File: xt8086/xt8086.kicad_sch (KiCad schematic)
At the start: 19 parts, among them J1 UART, J2 Ext Connector, J3 DEBUG, U1 SN74LS04, U2 SN74LS74

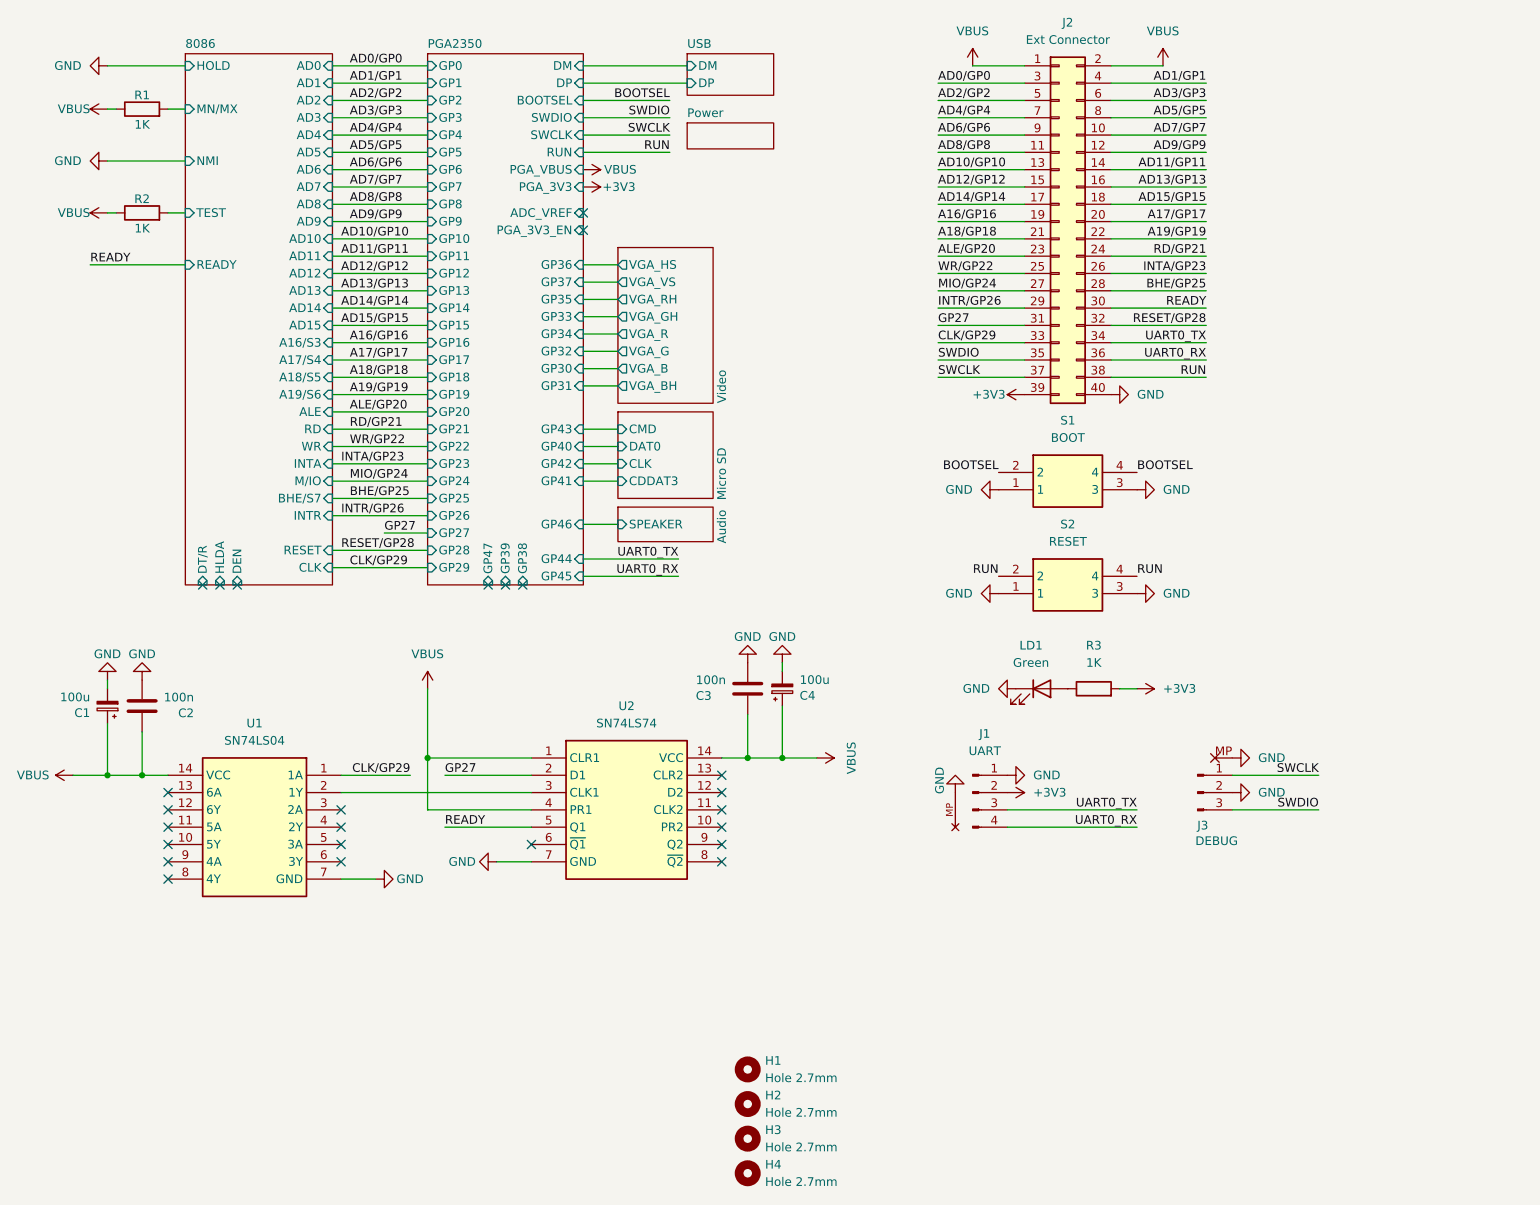
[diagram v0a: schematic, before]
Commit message: xt8086 WIP
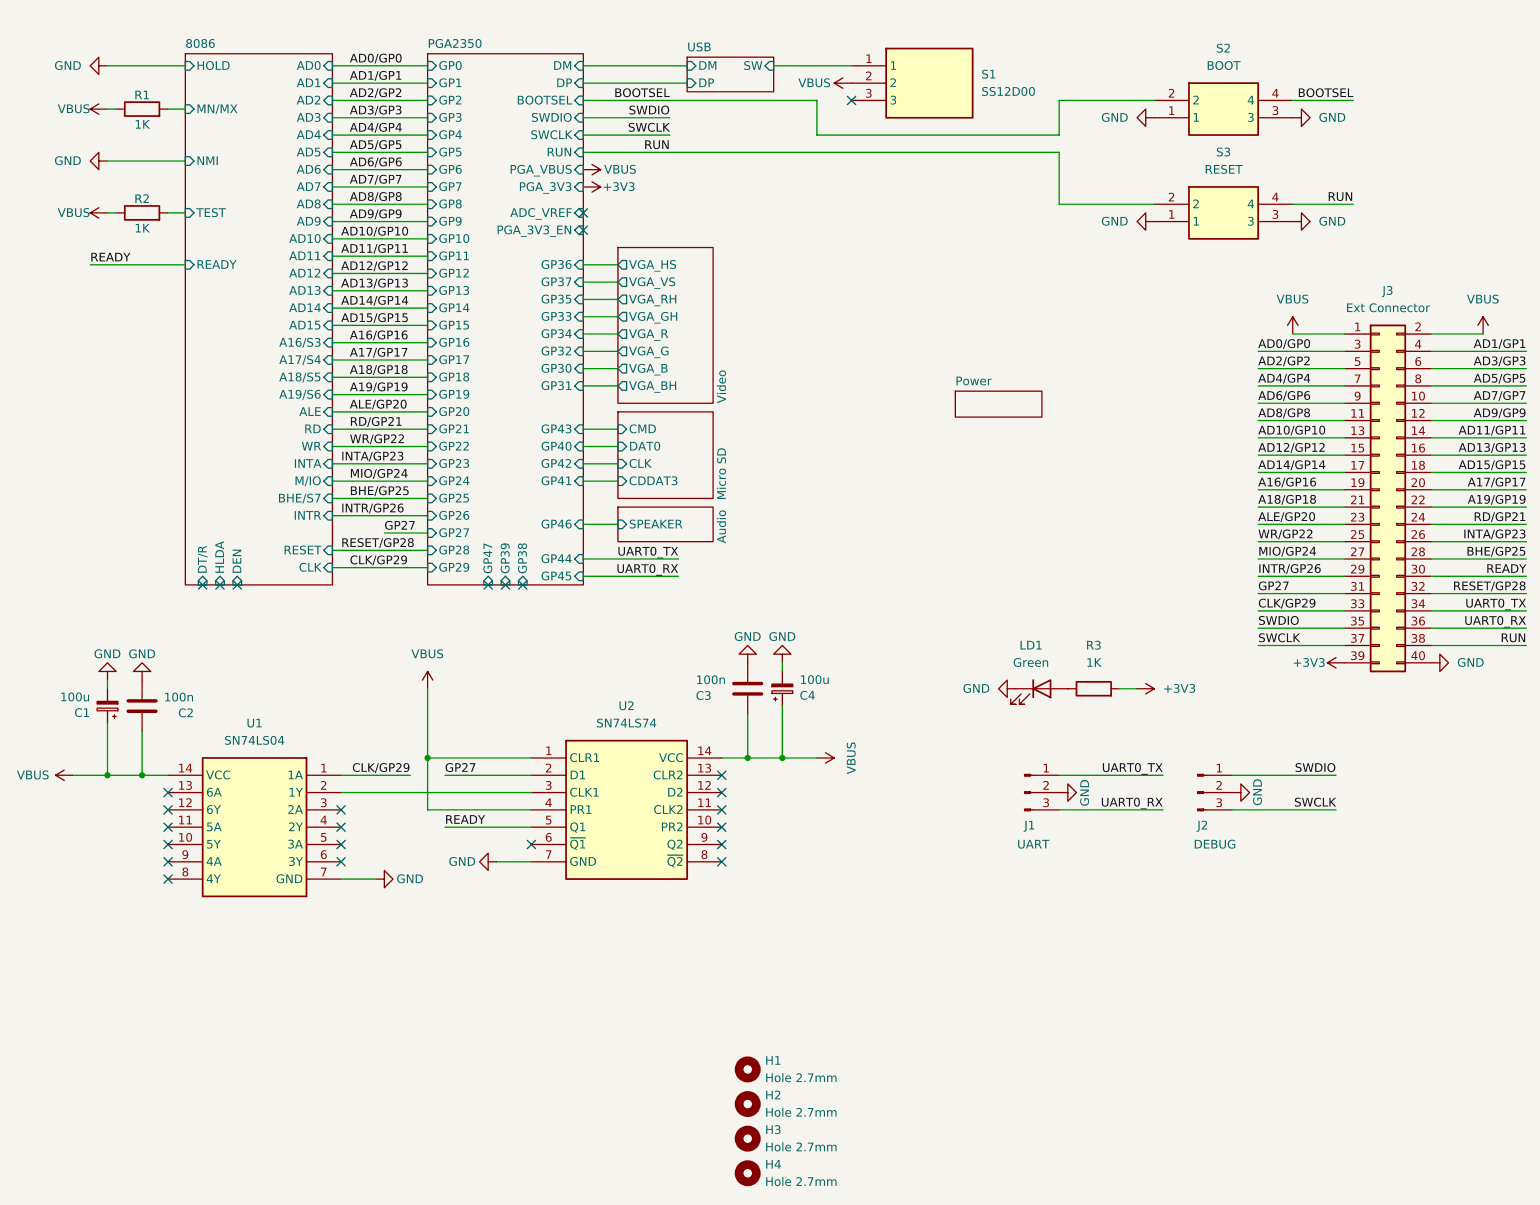
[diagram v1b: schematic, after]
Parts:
- removed J1: UART, xt8086:JST_SH_1x04_P1.00mm_Vertical, symbol xt8086:Conn_01x04_Pin
- added J1: UART, xt8086:JST_SH_1x03_P1.00mm_Vertical, symbol xt8086:Conn_01x03_Pin
- added S1: SS12D00, xt8086:Switch_Slide_SS12D00, symbol xt8086:SS12D00
- renumbered J3 to J2, J2 to J3, S1 to S2, S2 to S3
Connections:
- net GND: now also J1.2 (Pin_2); no longer J2.MP
- net SWCLK: now also J2.3 (Pin_3); no longer J2.1 (Pin_1)
- net SWDIO: now also J2.1 (Pin_1); no longer J2.3 (Pin_3)
- net UART0_RX: now also J1.3 (Pin_3)
- net UART0_TX: now also J1.1 (Pin_1)
- net VBUS: now also S1.2
- new net USB/SW: S1.1
- no-connect marks 25 -> 26
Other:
- sheet USB ports: added SW; removed none
- moved on the sheet: J3, S2, S3
